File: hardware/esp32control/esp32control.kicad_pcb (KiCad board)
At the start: 2 copper layers, 67.6 x 85.9 mm, 86 parts, among them J1 Conn_02x10_Odd_Even, Q1 BSS138, Q2 BSS138, Q3 BSS138, Q4 BSS138, Q5 BSS138, Q6 BSS138, Q7 MMBT3904, Q8 MMBT3904, SW1 Boot, SW2 Reset, U1 ESP32-WROOM, U10 LTV-354T, U11 HUT4, U12 LM1117-3.3, U13 RV-8523-C3, U2 AQY212, U3 AQY212, U4 LM2675M-5, U5 LTV-354T, U6 AQY212, U7 AQY212, U8 LTV-354T, U9 LTV-354T

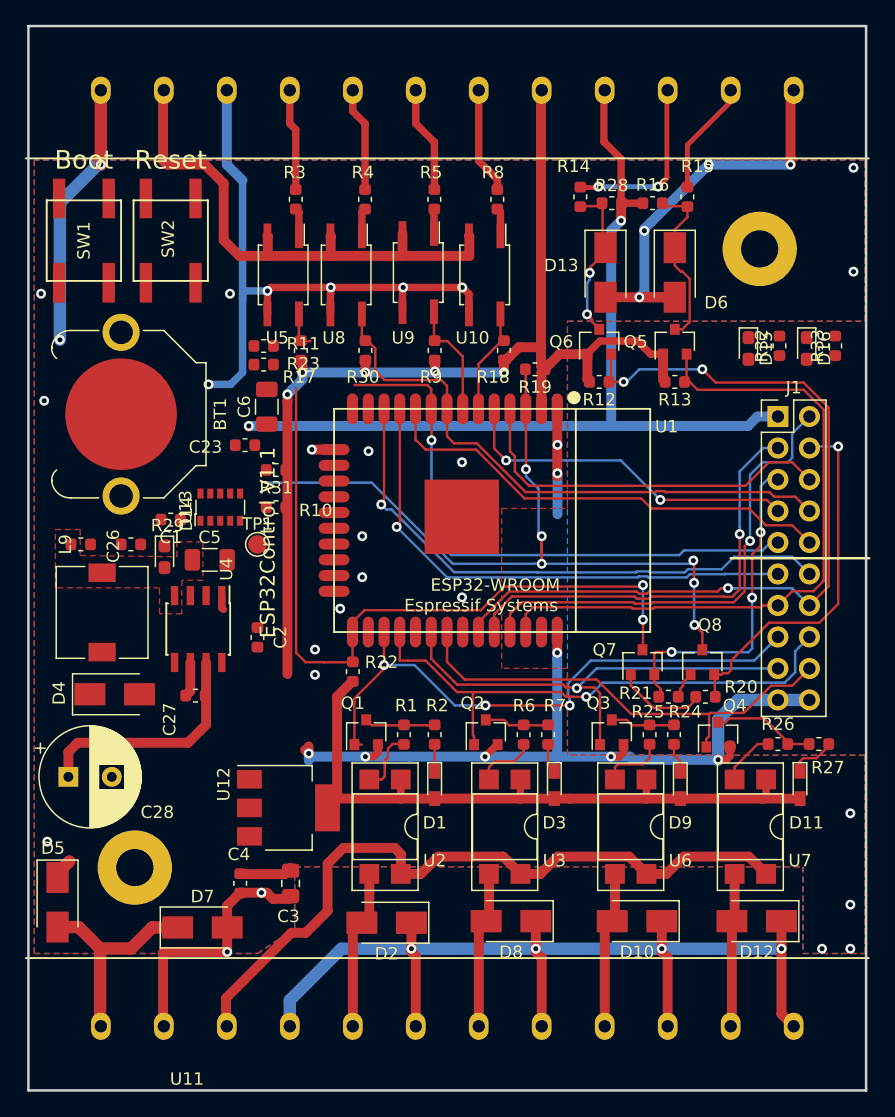
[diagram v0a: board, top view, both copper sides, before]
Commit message: pcb update, fab generated
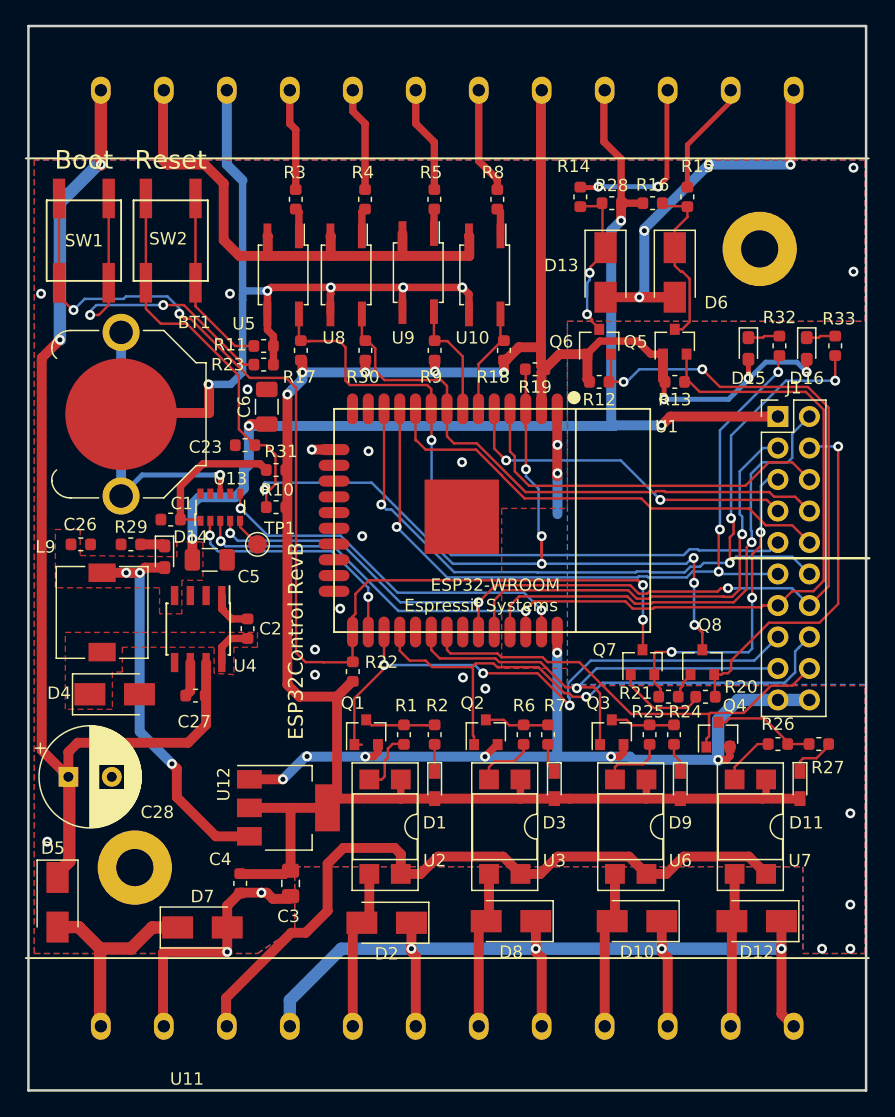
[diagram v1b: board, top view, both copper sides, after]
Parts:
- moved C2 1.06 mm to (69.2, 84.8)
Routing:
- net +5V: track 73.0 -> 121.7 mm, vias 2 -> 7
- net +24V: track 42.4 -> 86.0 mm
- net +3V3: track 149.8 -> 183.8 mm, vias 5 -> 8
- net /nBoot: track 59.4 -> 92.1 mm, vias 2 -> 4
- net /nReset: track 62.6 -> 95.2 mm, vias 6 -> 7
- net /IO23: track 0.00 -> 30.6 mm, vias 0 -> 2
- net /SCL: track 55.0 -> 83.8 mm, vias 0 -> 2
- net Net-(R23-Pad1): track 0.00 -> 26.1 mm, vias 0 -> 2
- net /SDA: track 67.7 -> 92.4 mm, vias 3 -> 5
- net Net-(BT1-Pad1): track 0.00 -> 23.4 mm, vias 0 -> 1
- net /IO27: track 45.8 -> 68.5 mm, vias 1 -> 4
- net /IO4: track 0.00 -> 19.7 mm, vias 0 -> 2
- net /IO26: track 42.2 -> 61.9 mm, vias 1 -> 4
- net GND: track 186.0 -> 203.7 mm, vias 38 -> 39
- net Net-(R11-Pad1): track 0.00 -> 14.7 mm
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- added copper zone on F.Cu, net Net-(C2-Pad2)
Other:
- rule trace_min: 0.15 -> 0.2
- board text added: "ESP32Control RevB"
- board text removed: "ESP32Control V1.1"
